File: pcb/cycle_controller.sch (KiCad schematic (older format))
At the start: 41 parts

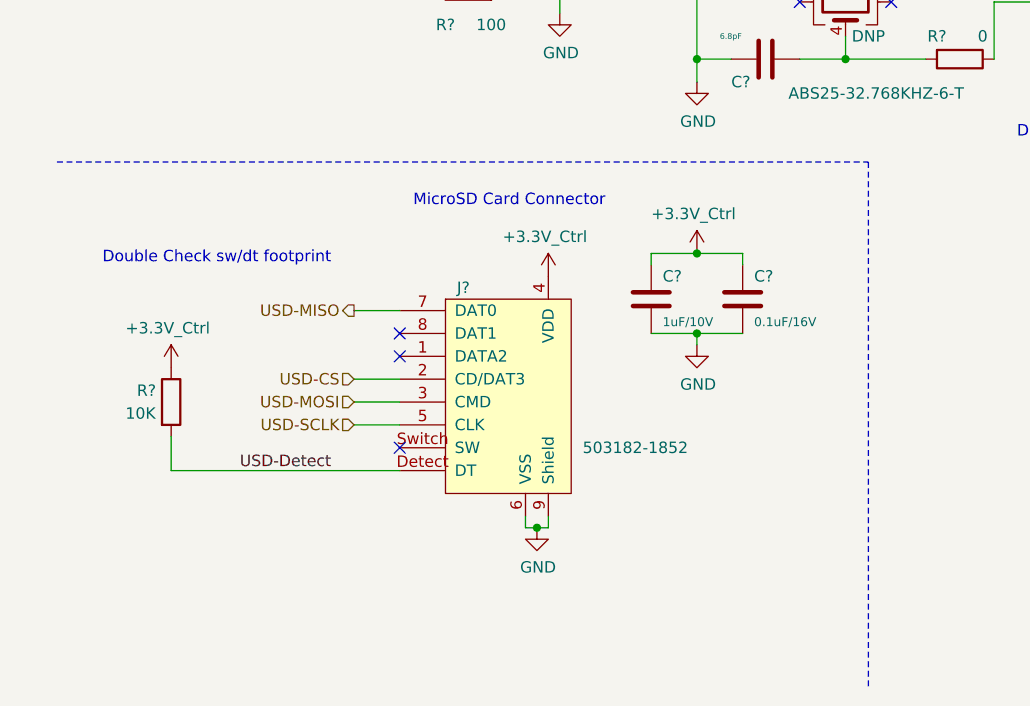
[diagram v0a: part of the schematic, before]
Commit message: ui computer
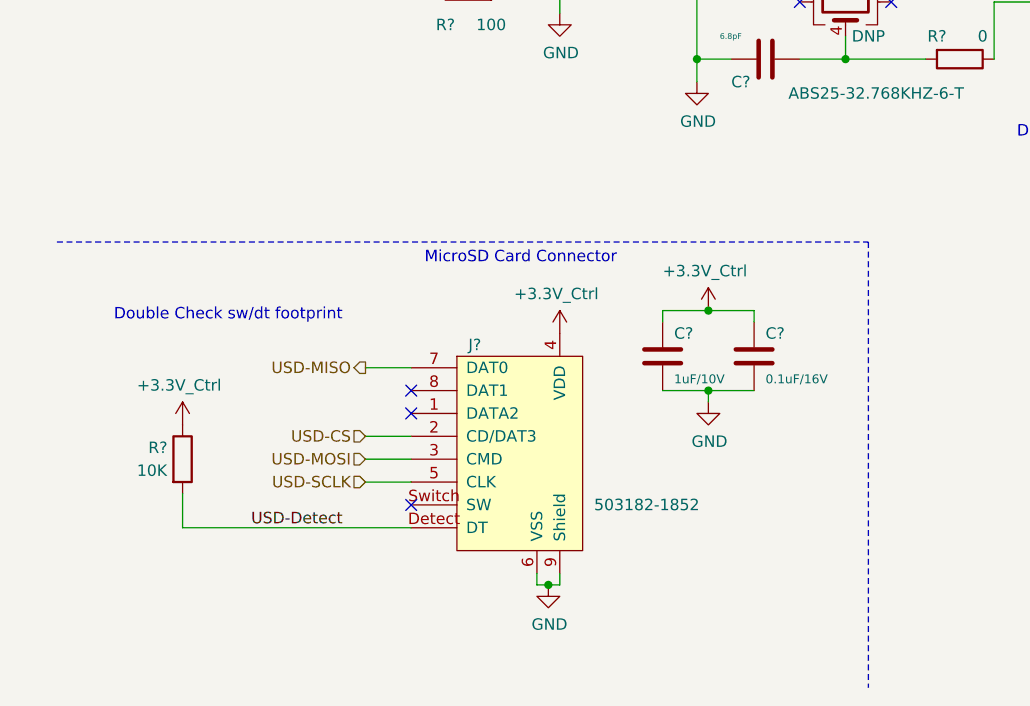
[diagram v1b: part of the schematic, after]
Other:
- moved on the sheet: C?, J?, R?
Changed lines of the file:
@@
 L RespiraWorks:503182-1852 J?
 U 1 1 6016937E
-P 2450 6400
+P 2500 6650
 AR Path="/5FCD4D4C/6016937E" Ref="J?"  Part="1"
 AR Path="/5FCD4D18/6016937E" Ref="J?"  Part="1"
-F 0 "J?" H 2250 6750 50  0000 L CNN
-F 1 "503182-1852" H 2800 6050 50  0000 L CNN
-F 2 "RespiraWorks:5031821852" H 3250 6000 50  0001 C CNN
-F 3 "https://www.molex.com/pdm_docs/sd/5031821852_sd.pdf" H 3850 5900 50  0001 C CNN
-	1    2450 6400
+F 0 "J?" H 2300 7000 50  0000 L CNN
+F 1 "503182-1852" H 2850 6300 50  0000 L CNN
+F 2 "RespiraWorks:5031821852" H 3300 6250 50  0001 C CNN
+F 3 "https://www.molex.com/pdm_docs/sd/5031821852_sd.pdf" H 3900 6150 50  0001 C CNN
+	1    2500 6650
 	1    0    0    -1
 $EndComp
-Text Notes 2900 5700 2    50   ~ 0
+Text Notes 2950 5950 2    50   ~ 0
 MicroSD Card Connector
 $Comp
 L RespiraWorks:+3.3V_Ctrl #PWR?
 U 1 1 60169386
-P 2650 6000
+P 2700 6250
 AR Path="/5FCD4D4C/60169386" Ref="#PWR?"  Part="1"
 AR Path="/5FCD4D18/60169386" Ref="#PWR?"  Part="1"
-F 0 "#PWR?" H 2650 6000 50  0001 C CNN
-F 1 "+3.3V_Ctrl" H 2635 6173 50  0000 C CNN
-F 2 "" H 2650 6000 50  0001 C CNN
-F 3 "" H 2650 6000 50  0001 C CNN
-	1    2650 6000
+F 0 "#PWR?" H 2700 6250 50  0001 C CNN
+F 1 "+3.3V_Ctrl" H 2685 6423 50  0000 C CNN
+F 2 "" H 2700 6250 50  0001 C CNN
+F 3 "" H 2700 6250 50  0001 C CNN
+	1    2700 6250
 	1    0    0    -1
 $EndComp
@@
 L Device:C C?
 U 1 1 6016938C
-P 3100 6100
+P 3150 6350
 AR Path="/5FCD4D4C/6016938C" Ref="C?"  Part="1"
 AR Path="/5FCD4D18/6016938C" Ref="C?"  Part="1"
-F 0 "C?" H 3150 6200 50  0000 L CNN
-F 1 "1uF/10V" H 3150 6000 39  0000 L CNN
-F 2 "" H 3138 5950 50  0001 C CNN
-F 3 "~" H 3100 6100 50  0001 C CNN
-	1    3100 6100
+F 0 "C?" H 3200 6450 50  0000 L CNN
+F 1 "1uF/10V" H 3200 6250 39  0000 L CNN
+F 2 "" H 3188 6200 50  0001 C CNN
+F 3 "~" H 3150 6350 50  0001 C CNN
+	1    3150 6350
 	1    0    0    -1
 $EndComp
@@
 L Device:C C?
 U 1 1 60169393
-P 3500 6100
+P 3550 6350
 AR Path="/5FCD4D4C/60169393" Ref="C?"  Part="1"
 AR Path="/5FCD4D18/60169393" Ref="C?"  Part="1"
-F 0 "C?" H 3550 6200 50  0000 L CNN
-F 1 "0.1uF/16V" H 3550 6000 39  0000 L CNN
-F 2 "" H 3538 5950 50  0001 C CNN
-F 3 "~" H 3500 6100 50  0001 C CNN
-	1    3500 6100
+F 0 "C?" H 3600 6450 50  0000 L CNN
+F 1 "0.1uF/16V" H 3600 6250 39  0000 L CNN
+F 2 "" H 3588 6200 50  0001 C CNN
+F 3 "~" H 3550 6350 50  0001 C CNN
+	1    3550 6350
 	1    0    0    -1
 $EndComp
@@
 L RespiraWorks:+3.3V_Ctrl #PWR?
 U 1 1 6016939A
-P 3300 5900
+P 3350 6150
 AR Path="/5FCD4D4C/6016939A" Ref="#PWR?"  Part="1"
 AR Path="/5FCD4D18/6016939A" Ref="#PWR?"  Part="1"
-F 0 "#PWR?" H 3300 5900 50  0001 C CNN
-F 1 "+3.3V_Ctrl" H 3285 6073 50  0000 C CNN
-F 2 "" H 3300 5900 50  0001 C CNN
-F 3 "" H 3300 5900 50  0001 C CNN
-	1    3300 5900
+F 0 "#PWR?" H 3350 6150 50  0001 C CNN
+F 1 "+3.3V_Ctrl" H 3335 6323 50  0000 C CNN
+F 2 "" H 3350 6150 50  0001 C CNN
+F 3 "" H 3350 6150 50  0001 C CNN
+	1    3350 6150
 	1    0    0    -1
 $EndComp
 Wire Wire Line
-	3100 5950 3100 5900
+	3150 6200 3150 6150
 Wire Wire Line
-	3100 5900 3300 5900
+	3150 6150 3350 6150
 Wire Wire Line
-	3300 5900 3500 5900
+	3350 6150 3550 6150
 Wire Wire Line
-	3500 5900 3500 5950
-Connection ~ 3300 5900
+	3550 6150 3550 6200
+Connection ~ 3350 6150
 $Comp
 L power:GND #PWR?
 U 1 1 601693A5
-P 3300 6300
+P 3350 6550
 AR Path="/5FCD4D4C/601693A5" Ref="#PWR?"  Part="1"
 AR Path="/5FCD4D18/601693A5" Ref="#PWR?"  Part="1"
-F 0 "#PWR?" H 3300 6050 50  0001 C CNN
-F 1 "GND" H 3305 6127 50  0000 C CNN
-F 2 "" H 3300 6300 50  0001 C CNN
-F 3 "" H 3300 6300 50  0001 C CNN
-	1    3300 6300
+F 0 "#PWR?" H 3350 6300 50  0001 C CNN
+F 1 "GND" H 3355 6377 50  0000 C CNN
+F 2 "" H 3350 6550 50  0001 C CNN
+F 3 "" H 3350 6550 50  0001 C CNN
+	1    3350 6550
 	1    0    0    -1
 $EndComp
 Wire Wire Line
-	3100 6250 3300 6250
+	3150 6500 3350 6500
 Wire Wire Line
-	3300 6250 3300 6300
+	3350 6500 3350 6550
 Wire Wire Line
-	3500 6250 3300 6250
-Connection ~ 3300 6250
+	3550 6500 3350 6500
+Connection ~ 3350 6500
 $Comp
 L power:GND #PWR?
 U 1 1 601693AF
-P 2600 7100
+P 2650 7350
 AR Path="/5FCD4D4C/601693AF" Ref="#PWR?"  Part="1"
 AR Path="/5FCD4D18/601693AF" Ref="#PWR?"  Part="1"
-F 0 "#PWR?" H 2600 6850 50  0001 C CNN
-F 1 "GND" H 2605 6927 50  0000 C CNN
-F 2 "" H 2600 7100 50  0001 C CNN
-F 3 "" H 2600 7100 50  0001 C CNN
-	1    2600 7100
+F 0 "#PWR?" H 2650 7100 50  0001 C CNN
+F 1 "GND" H 2655 7177 50  0000 C CNN
+F 2 "" H 2650 7350 50  0001 C CNN
+F 3 "" H 2650 7350 50  0001 C CNN
+	1    2650 7350
 	1    0    0    -1
 $EndComp
 Wire Wire Line
-	2600 7100 2650 7100
+	2650 7350 2700 7350
 Wire Wire Line
-	2650 7100 2650 7050
+	2700 7350 2700 7300
 Wire Wire Line
-	2550 7050 2550 7100
+	2600 7300 2600 7350
 Wire Wire Line
-	2550 7100 2600 7100
-Connection ~ 2600 7100
-Text Notes 1700 5950 2    50   ~ 0
+	2600 7350 2650 7350
+Connection ~ 2650 7350
+Text Notes 1750 6200 2    50   ~ 0
 Double Check sw/dt footprint
-NoConn ~ 2000 6250
-NoConn ~ 2000 6350
-NoConn ~ 2000 6750
-Text Label 1700 6850 2    50   ~ 0
+NoConn ~ 2050 6500
+NoConn ~ 2050 6600
+NoConn ~ 2050 7000
+Text Label 1750 7100 2    50   ~ 0
 USD-Detect
 Wire Wire Line
-	1000 6850 2000 6850
+	1050 7100 2050 7100
 Wire Wire Line
-	1000 6850 1000 6700
+	1050 7100 1050 6950
 $Comp
 L Device:R R?
 U 1 1 601693C1
-P 1000 6550
+P 1050 6800
 AR Path="/5FCD4D4C/601693C1" Ref="R?"  Part="1"
 AR Path="/5FCD4D18/601693C1" Ref="R?"  Part="1"
-F 0 "R?" H 850 6600 50  0000 L CNN
-F 1 "10K" H 800 6500 50  0000 L CNN
-F 2 "RespiraWorks_std:R_0603_1608Metric" V 930 6550 50  0001 C CNN
-F 3 "~" H 1000 6550 50  0001 C CNN
-	1    1000 6550
+F 0 "R?" H 900 6850 50  0000 L CNN
+F 1 "10K" H 850 6750 50  0000 L CNN
+F 2 "RespiraWorks_std:R_0603_1608Metric" V 980 6800 50  0001 C CNN
+F 3 "~" H 1050 6800 50  0001 C CNN
+	1    1050 6800
 	1    0    0    -1
 $EndComp
@@
 L RespiraWorks:+3.3V_Ctrl #PWR?
 U 1 1 601693C8
-P 1000 6400
+P 1050 6650
 AR Path="/5FCD4D4C/601693C8" Ref="#PWR?"  Part="1"
 AR Path="/5FCD4D18/601693C8" Ref="#PWR?"  Part="1"
-F 0 "#PWR?" H 1000 6400 50  0001 C CNN
-F 1 "+3.3V_Ctrl" H 985 6573 50  0000 C CNN
-F 2 "" H 1000 6400 50  0001 C CNN
-F 3 "" H 1000 6400 50  0001 C CNN
-	1    1000 6400
+F 0 "#PWR?" H 1050 6650 50  0001 C CNN
+F 1 "+3.3V_Ctrl" H 1035 6823 50  0000 C CNN
+F 2 "" H 1050 6650 50  0001 C CNN
+F 3 "" H 1050 6650 50  0001 C CNN
+	1    1050 6650
 	1    0    0    -1
 $EndComp
 Wire Wire Line
-	2000 6650 1800 6650
+	2050 6900 1850 6900
 Wire Wire Line
-	2000 6550 1800 6550
+	2050 6800 1850 6800
 Wire Wire Line
-	2000 6450 1800 6450
+	2050 6700 1850 6700
 Wire Wire Line
-	2000 6150 1800 6150
-Text HLabel 1800 6150 0    50   Output ~ 0
+	2050 6400 1850 6400
+Text HLabel 1850 6400 0    50   Output ~ 0
 USD-MISO
-Text HLabel 1800 6450 0    50   Input ~ 0
+Text HLabel 1850 6700 0    50   Input ~ 0
 USD-CS
-Text HLabel 1800 6550 0    50   Input ~ 0
+Text HLabel 1850 6800 0    50   Input ~ 0
 USD-MOSI
-Text HLabel 1800 6650 0    50   Input ~ 0
+Text HLabel 1850 6900 0    50   Input ~ 0
 USD-SCLK
 Wire Notes Line
-	500  5500 4050 5500
+	500  5850 4050 5850
 Wire Notes Line
-	4050 5500 4050 7800
+	4050 5850 4050 7800
 NoConn ~ 6400 1600
 Wire Wire Line
